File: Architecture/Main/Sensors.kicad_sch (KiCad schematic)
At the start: 5 parts, among them J2 Screw_Terminal_01x02, J4 Conn_01x04, J6 Conn_01x04

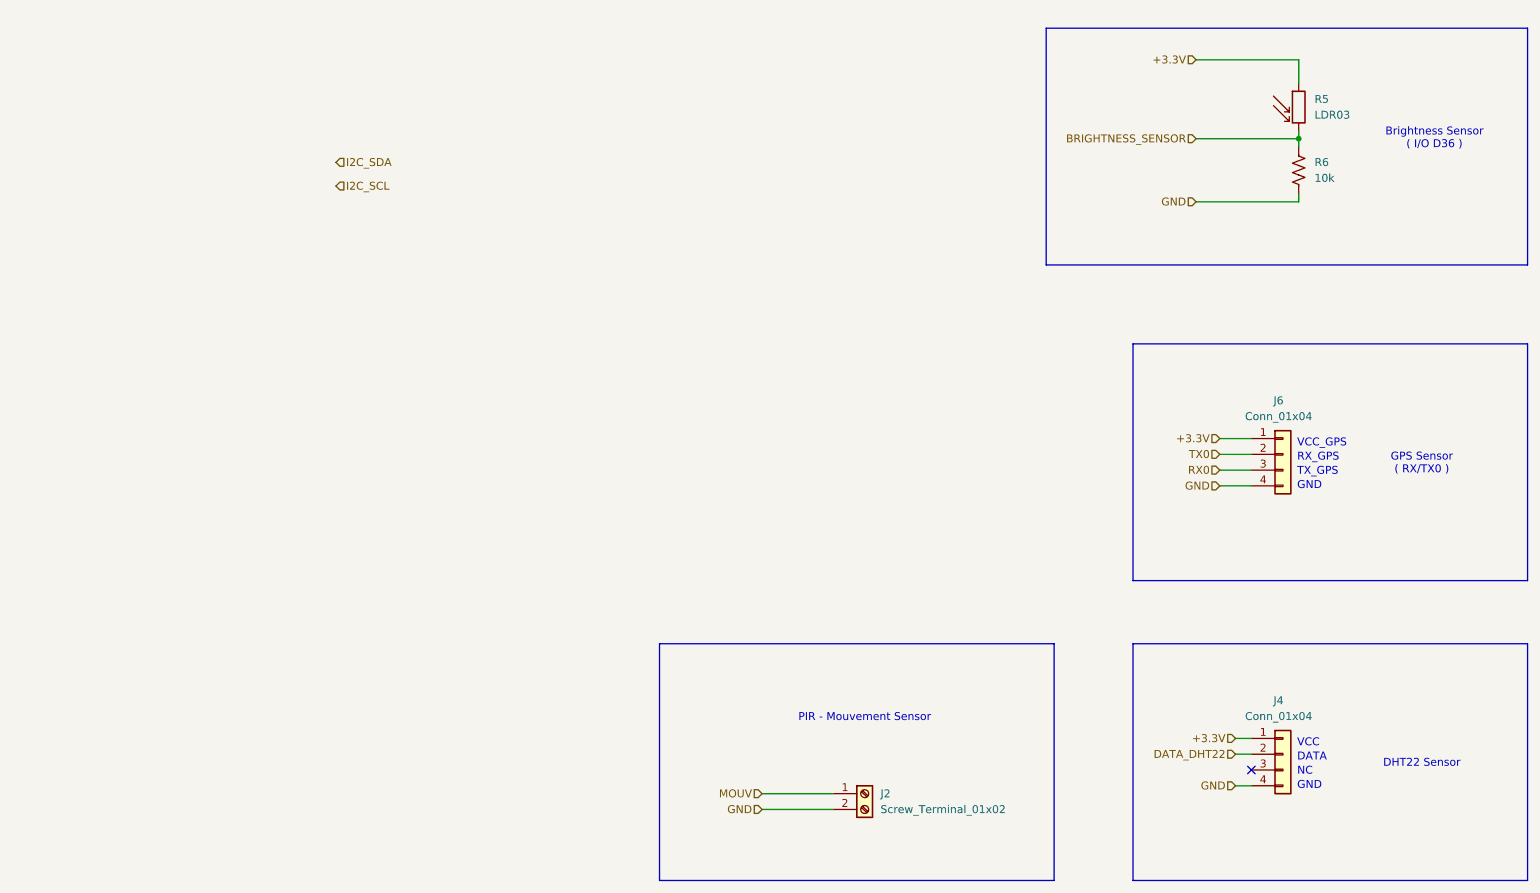
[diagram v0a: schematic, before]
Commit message: update
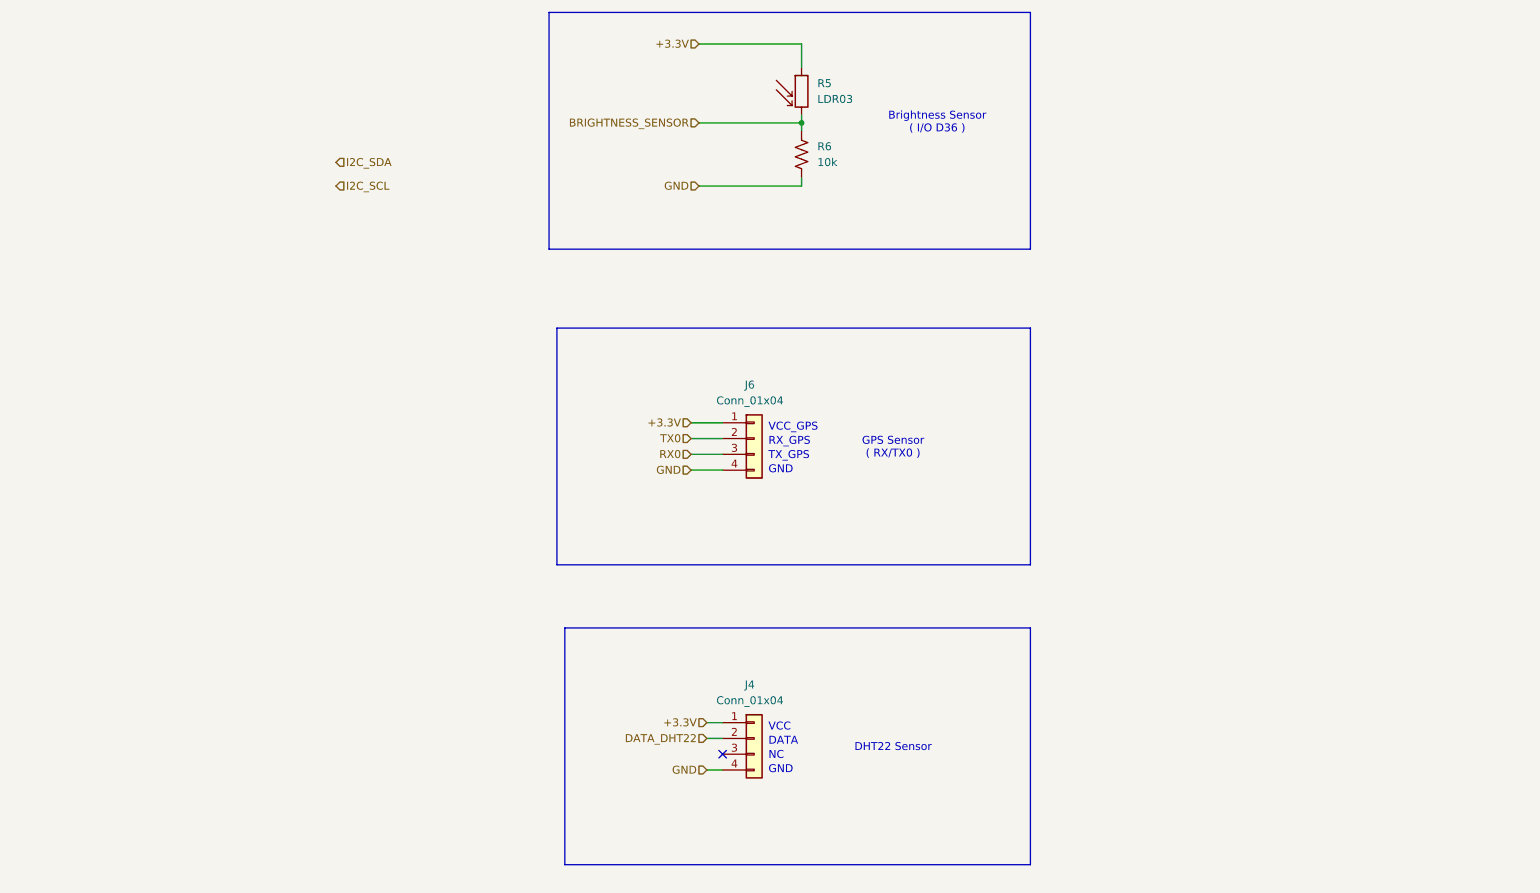
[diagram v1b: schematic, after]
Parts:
- removed J2: Screw_Terminal_01x02, symbol Connector:Screw_Terminal_01x02
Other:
- note removed: "PIR - Mouvement Sensor"
- moved on the sheet: J4, J6, R5, R6

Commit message: Update_07_01_2026
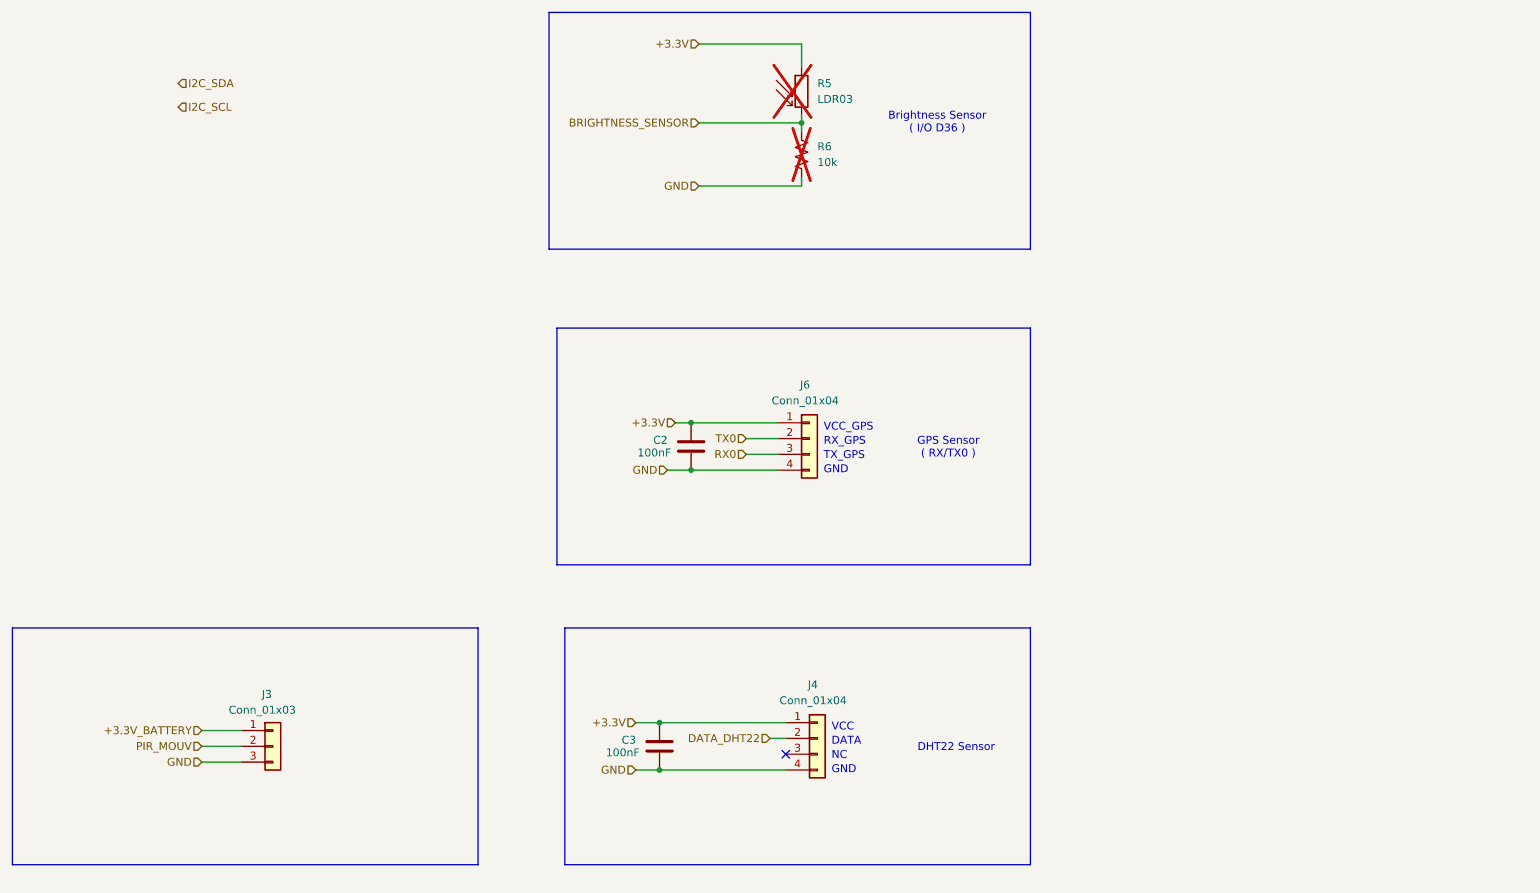
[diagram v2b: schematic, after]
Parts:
- added C2, C3: 100nF, symbol Device:C
- added J3: Conn_01x03, symbol Connector_Generic:Conn_01x03
- R5, R6: now not fitted; now left out of the parts list
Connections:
- net +3.3V: now also C2.1, C3.1
- net GND: now also C2.2, C3.2, J3.3 (Pin_3)
- new net +3.3V_BATTERY: J3.1 (Pin_1)
- new net PIR_MOUV: J3.2 (Pin_2)
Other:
- moved on the sheet: J4, J6
